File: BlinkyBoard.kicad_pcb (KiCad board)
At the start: 2 copper layers, 119.3 x 120.3 mm, 19 parts, among them J1 Conn_01x02_Socket, J2 Conn_01x02_Socket, U1 NE555P, U2 4017

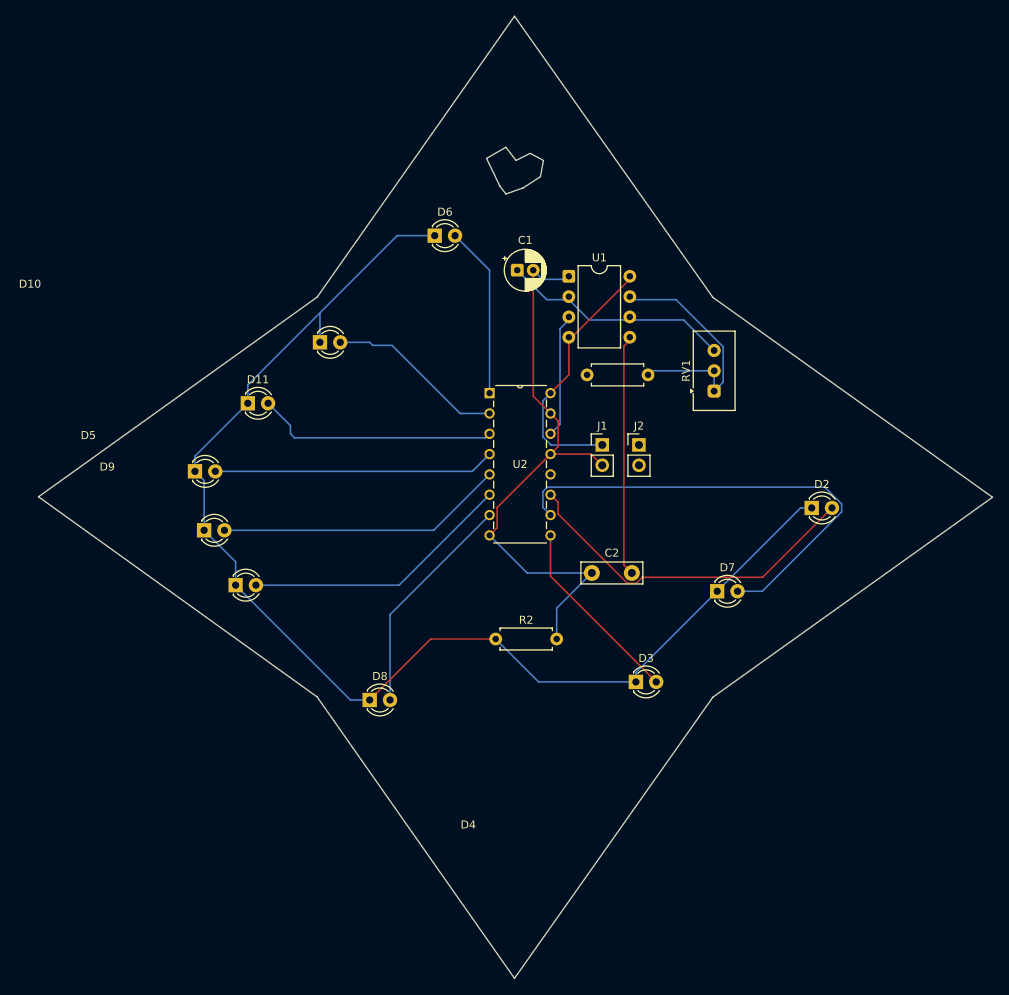
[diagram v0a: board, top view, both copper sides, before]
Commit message: final edits!
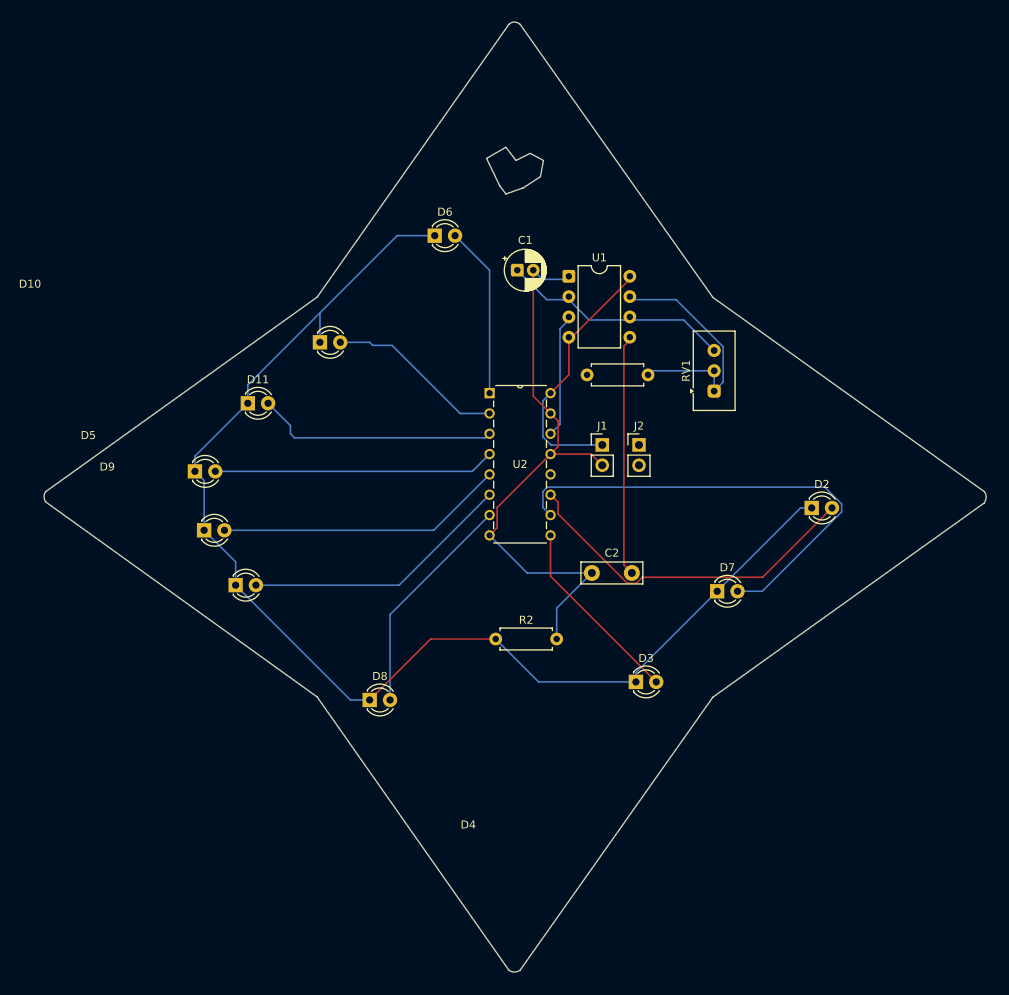
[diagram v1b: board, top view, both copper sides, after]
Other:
- board size 119.3 x 120.3 mm -> 117.8 x 118.7 mm
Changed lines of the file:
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@@
+		(layer "Edge.Cuts")
+	)
+	(gr_curve
+		(pts
+			(xy 70.739 124.714) (xy 70.2945 125.349) (xy 70.739 125.984) (xy 70.739 125.984)
+		)
+		(stroke
+			(width 0.05)
+			(type default)
+		)
 		(layer "Edge.Cuts")
 	)
 	(gr_line
-		(start 69.85 125.349)
+		(start 70.739 124.714)
 		(end 104.67975 100.3935)
 		(stroke
@@
 	)
 	(gr_line
-		(start 69.85 125.349)
+		(start 70.739 125.984)
 		(end 104.67975 150.368)
 		(stroke
@@
 	)
 	(gr_line
-		(start 104.67975 100.3935)
-		(end 129.3495 65.278)
+		(start 128.651 66.294)
+		(end 104.67975 100.3935)
+		(stroke
+			(width 0.05)
+			(type default)
+		)
+		(layer "Edge.Cuts")
+	)
+	(gr_curve
+		(pts
+			(xy 128.651 66.294) (xy 129.3495 65.659) (xy 130.048 66.294) (xy 130.048 66.294)
+		)
 		(stroke
 			(width 0.05)
@@
 	)
 	(gr_line
-		(start 129.3495 65.278)
+		(start 128.651 184.531)
+		(end 104.67975 150.368)
+		(stroke
+			(width 0.05)
+			(type default)
+		)
+		(layer "Edge.Cuts")
+	)
+	(gr_curve
+		(pts
+			(xy 128.651 184.531) (xy 129.3495 185.039) (xy 130.048 184.531) (xy 130.048 184.531)
+		)
+		(stroke
+			(width 0.05)
+			(type default)
+		)
+		(layer "Edge.Cuts")
+	)
+	(gr_line
+		(start 130.048 66.294)
 		(end 154.14625 100.42525)
 		(stroke
@@
 	)
 	(gr_line
-		(start 129.3495 185.547)
-		(end 104.67975 150.368)
-		(stroke
-			(width 0.05)
-			(type default)
-		)
-		(layer "Edge.Cuts")
-	)
-	(gr_line
-		(start 129.3495 185.547)
+		(start 130.048 184.531)
 		(end 154.14625 150.39975)
-		(stroke
-			(width 0.05)
-			(type default)
-		)
-		(layer "Edge.Cuts")
-	)
-	(gr_line
-		(start 154.14625 100.42525)
-		(end 189.103 125.4125)
 		(stroke
 			(width 0.05)
@@
 	)
 	(gr_line
-		(start 189.103 125.4125)
+		(start 188.087 124.714)
+		(end 154.14625 100.42525)
+		(stroke
+			(width 0.05)
+			(type default)
+		)
+		(layer "Edge.Cuts")
+	)
+	(gr_curve
+		(pts
+			(xy 188.087 124.714) (xy 188.595 125.4125) (xy 188.04819 126.111) (xy 188.087 126.111)
+		)
+		(stroke
+			(width 0.05)
+			(type default)
+		)
+		(layer "Edge.Cuts")
+	)
+	(gr_line
+		(start 188.087 126.111)
 		(end 154.14625 150.39975)
 		(stroke
 			(width 0.05)
+			(type default)
+		)
+		(layer "Edge.Cuts")
+	)
+	(gr_curve
+		(pts
+			(xy 188.087 126.111) (xy 188.087 126.111) (xy 188.087 126.111) (xy 188.087 126.111)
+		)
+		(stroke
+			(width 0.05)
